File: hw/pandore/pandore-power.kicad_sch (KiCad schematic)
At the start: 1 part, among them J6 VIN

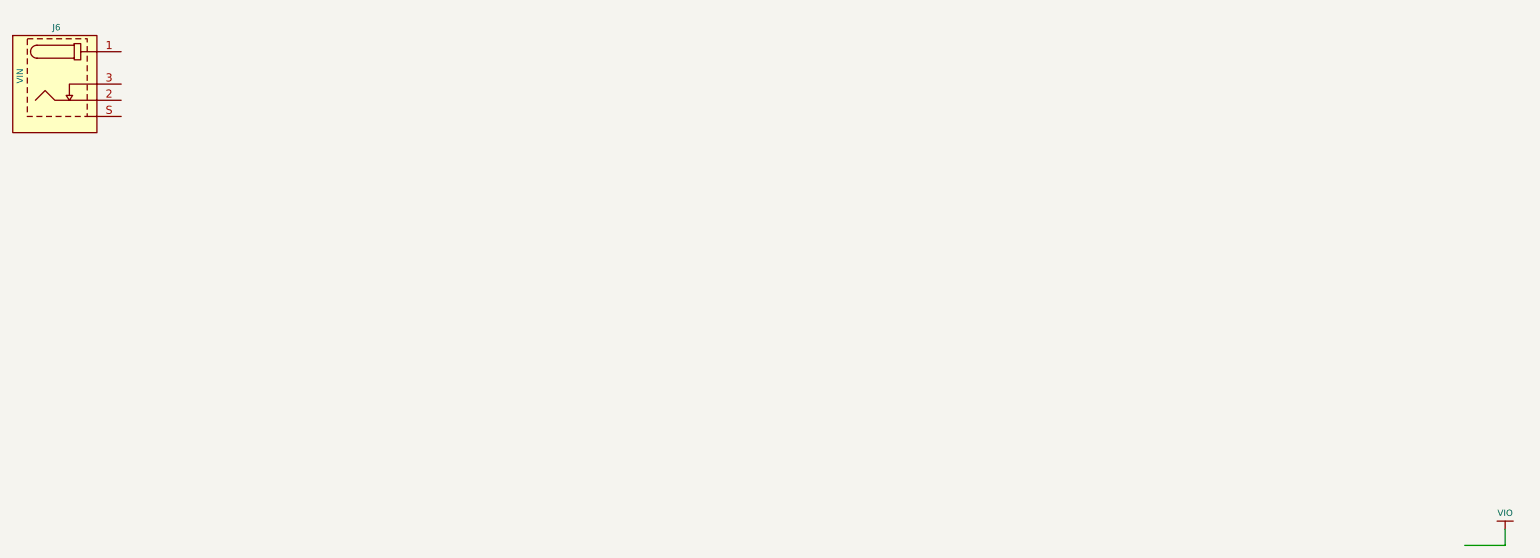
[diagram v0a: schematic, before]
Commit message: lots of work done all around
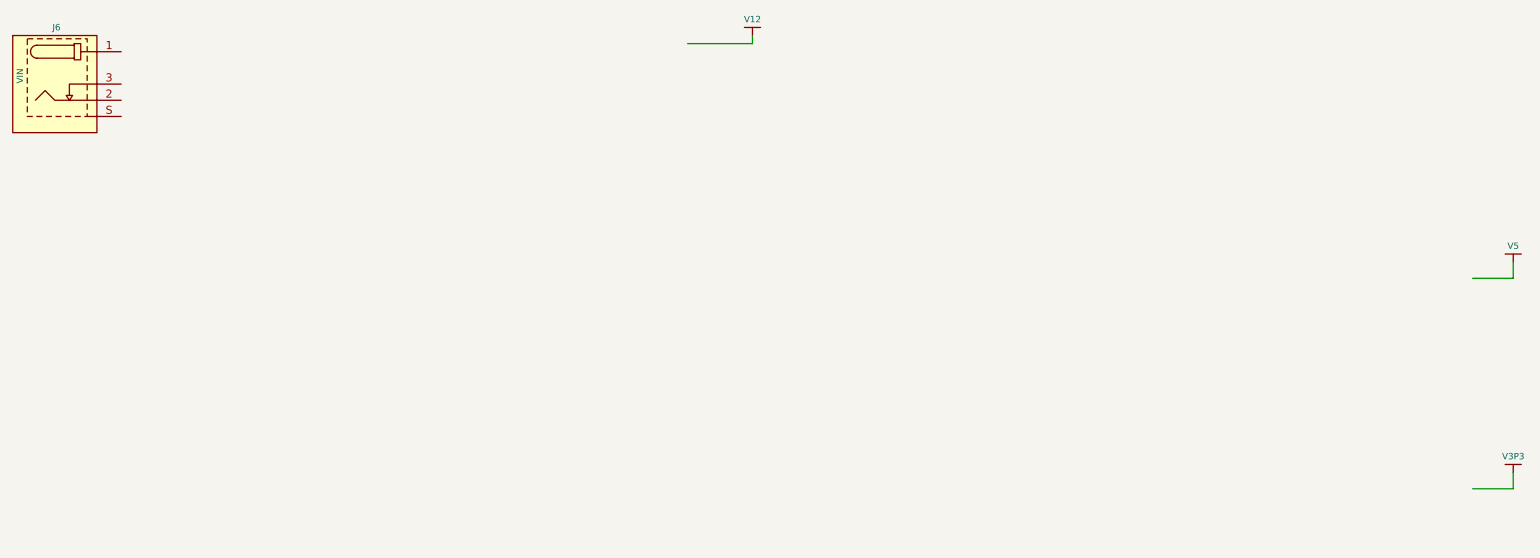
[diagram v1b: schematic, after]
